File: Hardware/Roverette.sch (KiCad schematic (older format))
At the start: 40 parts, among them SW1 SW_Push, U1 ESP32-WROOM-32U

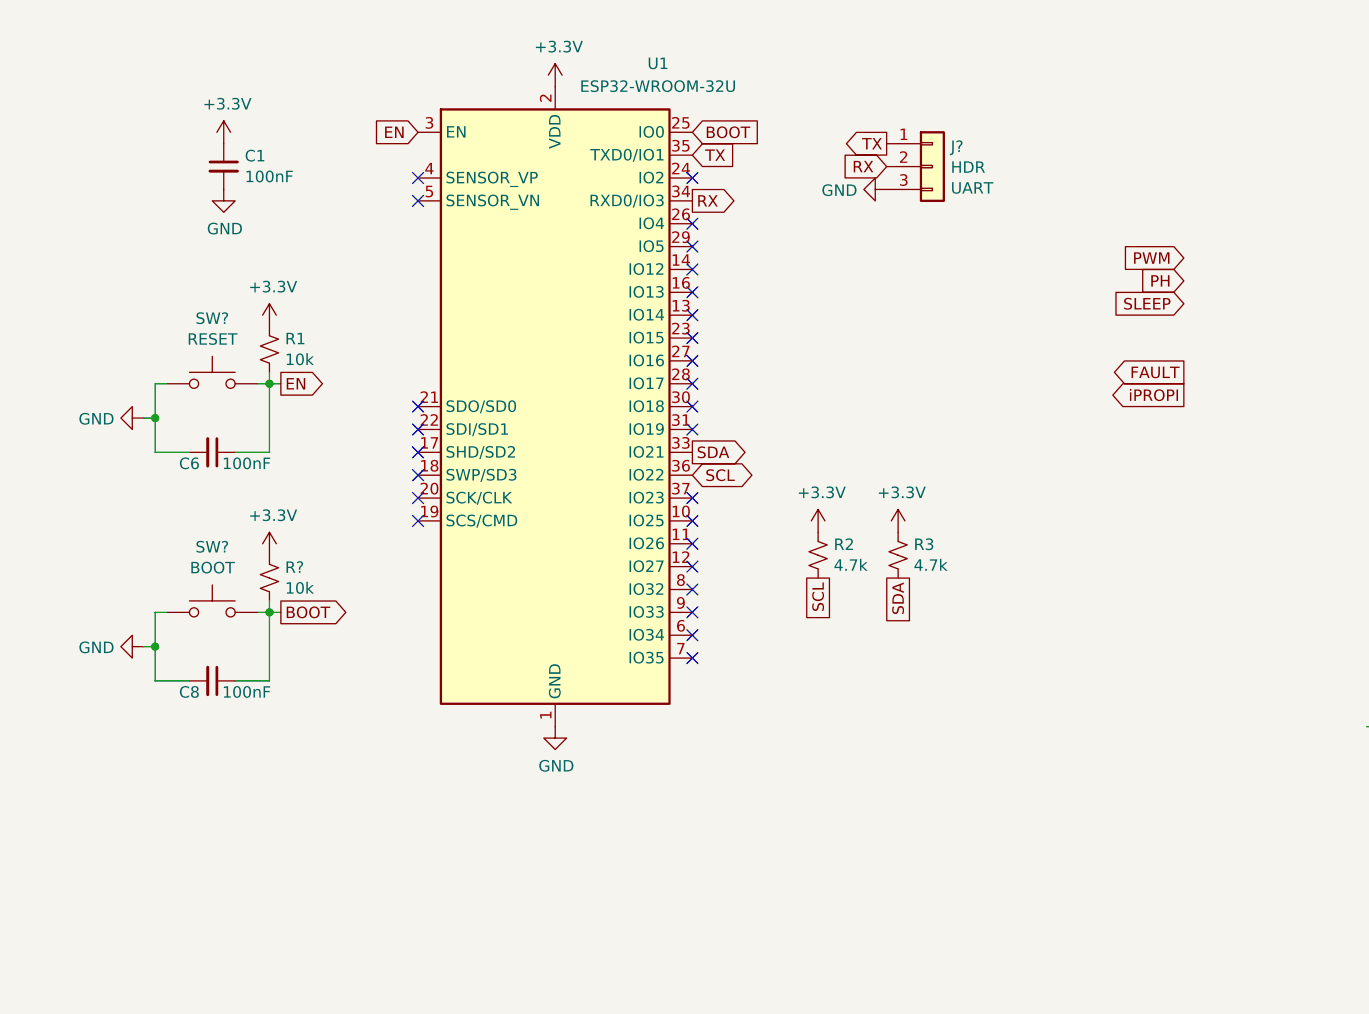
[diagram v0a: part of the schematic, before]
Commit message: Schematic updated
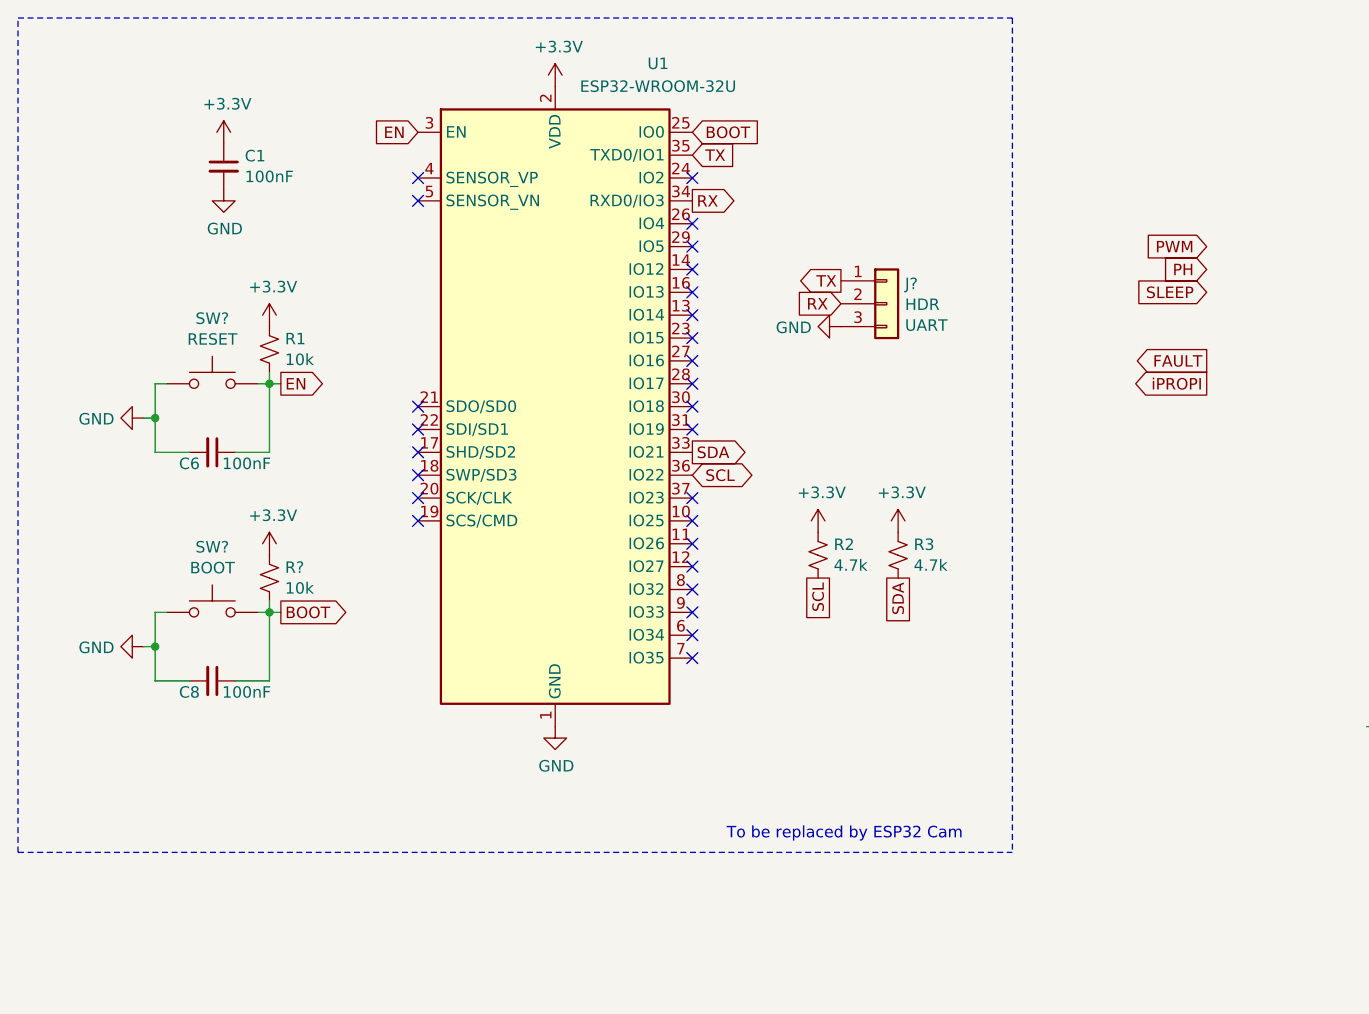
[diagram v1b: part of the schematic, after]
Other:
- note added: "To be replaced by ESP32 Cam"
- moved on the sheet: J?
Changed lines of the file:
@@
 NoConn ~ 4050 3500
 NoConn ~ 4050 3600
-Text GLabel 6200 2050 0    50   Input ~ 0
+Text GLabel 6300 2000 0    50   Input ~ 0
 PWM
-Text GLabel 6200 2150 0    50   Input ~ 0
+Text GLabel 6300 2100 0    50   Input ~ 0
 PH
-Text GLabel 6200 2250 0    50   Input ~ 0
+Text GLabel 6300 2200 0    50   Input ~ 0
 SLEEP
-Text GLabel 6200 2550 0    50   Output ~ 0
+Text GLabel 6300 2500 0    50   Output ~ 0
 FAULT
-Text GLabel 6200 2650 0    50   Output ~ 0
+Text GLabel 6300 2600 0    50   Output ~ 0
 iPROPI
 $Bitmap
@@
 L Connector_Generic:Conn_01x03 J?
 U 1 1 5FF13025
-P 5100 1650
-F 0 "J?" H 5180 1737 50  0000 L CNN
-F 1 "HDR" H 5180 1646 50  0000 L CNN
-F 2 "" H 5100 1650 50  0001 C CNN
-F 3 "~" H 5100 1650 50  0001 C CNN
-F 4 "UART" H 5180 1555 50  0000 L CNN "Field4"
-	1    5100 1650
+P 4900 2250
+F 0 "J?" H 4980 2337 50  0000 L CNN
+F 1 "HDR" H 4980 2246 50  0000 L CNN
+F 2 "" H 4900 2250 50  0001 C CNN
+F 3 "~" H 4900 2250 50  0001 C CNN
+F 4 "UART" H 4980 2155 50  0000 L CNN "Field4"
+	1    4900 2250
 	1    0    0    -1
 $EndComp
@@
 Text GLabel 4050 1600 2    50   Input ~ 0
 TX
-Text GLabel 4900 1650 0    50   Input ~ 0
+Text GLabel 4700 2250 0    50   Input ~ 0
 RX
-Text GLabel 4900 1550 0    50   Output ~ 0
+Text GLabel 4700 2150 0    50   Output ~ 0
 TX
 $Comp
 L power:GND #PWR?
 U 1 1 5FF3D9B5
-P 4900 1750
-F 0 "#PWR?" H 4900 1500 50  0001 C CNN
-F 1 "GND" V 4905 1622 50  0000 R CNN
-F 2 "" H 4900 1750 50  0001 C CNN
-F 3 "" H 4900 1750 50  0001 C CNN
-	1    4900 1750
+P 4700 2350
+F 0 "#PWR?" H 4700 2100 50  0001 C CNN
+F 1 "GND" V 4705 2222 50  0000 R CNN
+F 2 "" H 4700 2350 50  0001 C CNN
+F 3 "" H 4700 2350 50  0001 C CNN
+	1    4700 2350
 	0    1    1    0
 $EndComp
@@
 Wire Wire Line
 	1500 7000 2050 7000
+Wire Notes Line
+	1100 4650 1100 1000
+Wire Notes Line
+	1100 1000 5450 1000
+Wire Notes Line
+	5450 1000 5450 4650
+Wire Notes Line
+	1100 4650 5450 4650
+Text Notes 4200 4600 0    50   ~ 0
+To be replaced by ESP32 Cam
 $EndSCHEMATC
